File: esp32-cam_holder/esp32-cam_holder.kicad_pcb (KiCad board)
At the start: 2 copper layers, 28 x 55 mm, 6 parts, among them J1 RJ45_Shielded, J2 UART, U1 ESP32-CAM

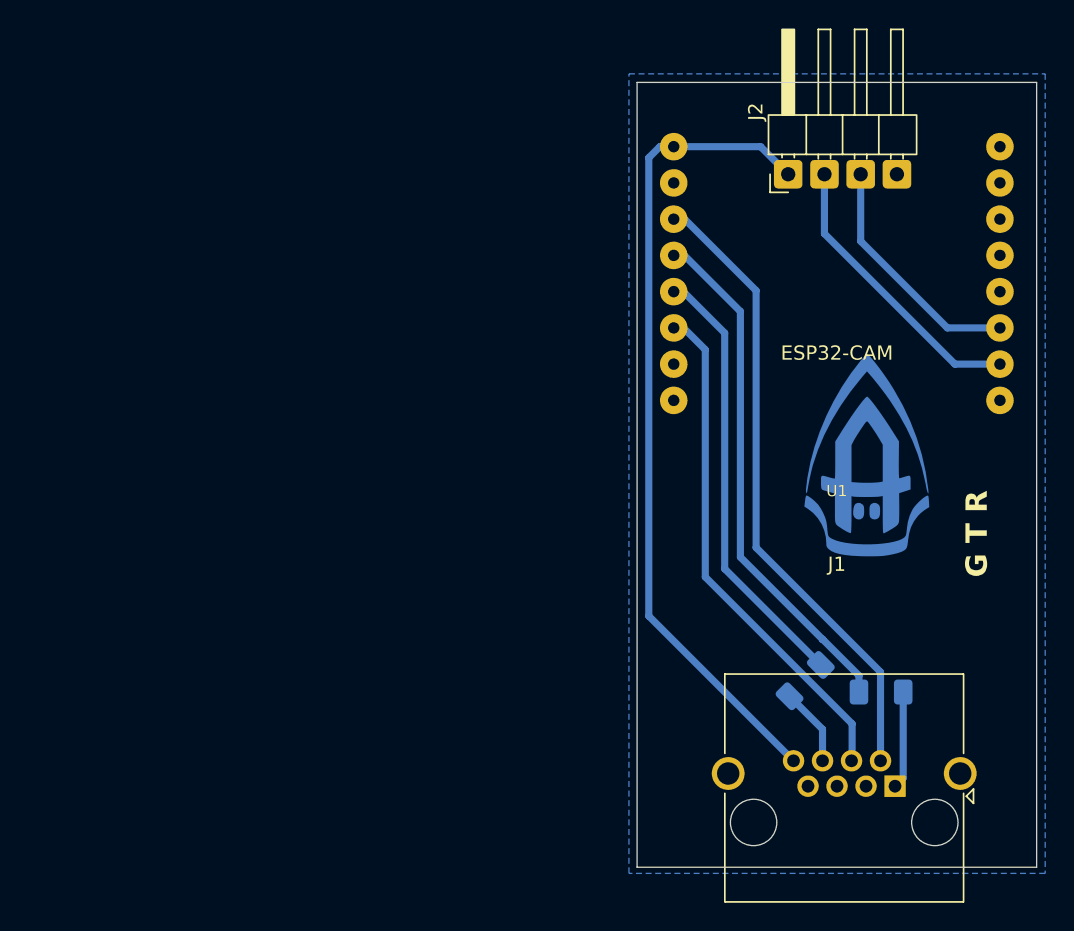
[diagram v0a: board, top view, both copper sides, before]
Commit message: REV ALL
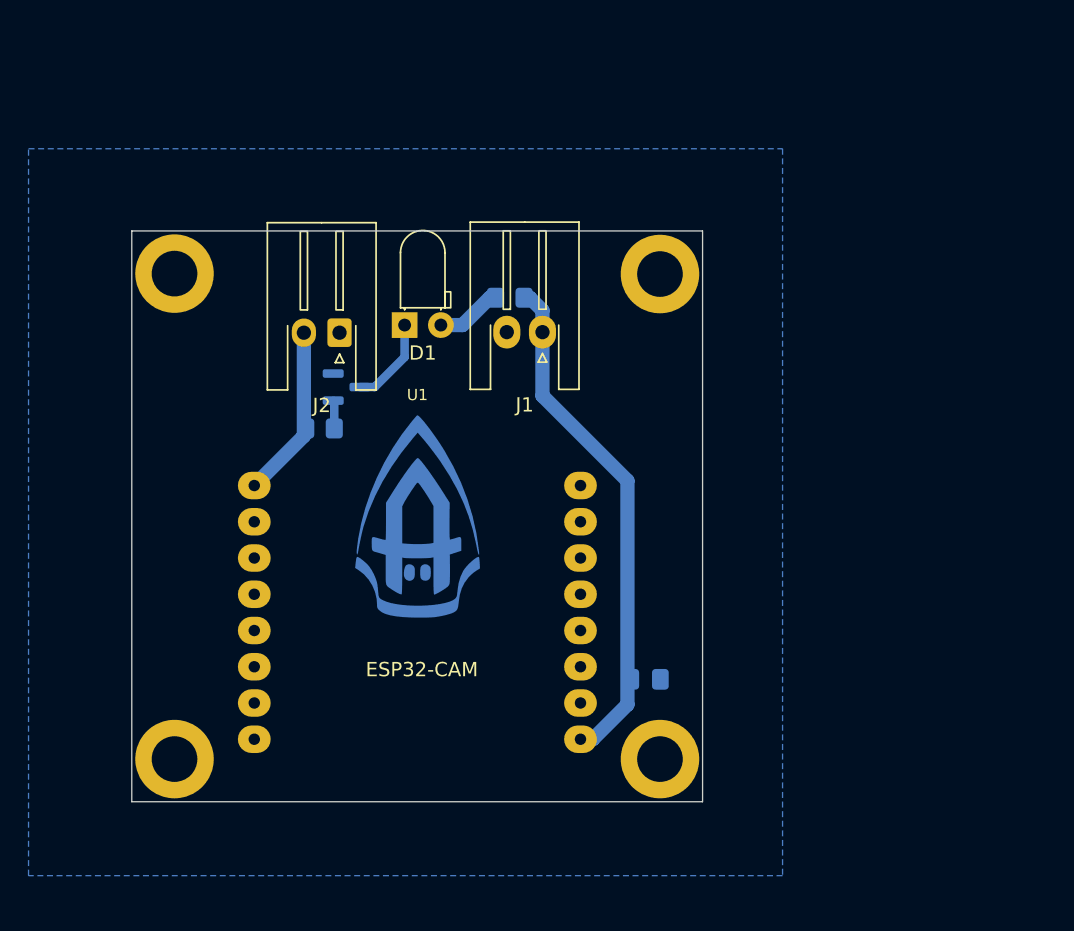
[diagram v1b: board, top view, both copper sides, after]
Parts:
- added C1: 100nF, Capacitor_SMD:C_0805_2012Metric_Pad1.18x1.45mm_HandSolder, B.Cu at (135.6, 57.1)
- added D1: LED, LED_THT:LED_D3.0mm_Horizontal_O1.27mm_Z6.0mm, F.Cu at (121.2, 32.3)
- added Q1: MMBT3904, Package_TO_SOT_SMD:SOT-23, B.Cu at (114.6, 36.7)
- added REF**: MountingHole_3.2mm_M3_ISO14580_Pad, MountingHole:MountingHole_3.2mm_M3_ISO14580_Pad, F.Cu at (102.6, 62.7)
- added REF**: MountingHole_3.2mm_M3_ISO14580_Pad, MountingHole:MountingHole_3.2mm_M3_ISO14580_Pad, F.Cu at (136.6, 62.7)
- added REF**: MountingHole_3.2mm_M3_ISO14580_Pad, MountingHole:MountingHole_3.2mm_M3_ISO14580_Pad, F.Cu at (136.6, 28.7)
- added REF**: MountingHole_3.2mm_M3_ISO14580_Pad, MountingHole:MountingHole_3.2mm_M3_ISO14580_Pad, F.Cu at (102.6, 28.7)
- J1: value RJ45_Shielded -> power; footprint Connector_RJ:RJ45_Amphenol_RJHSE5380 -> Connector_JST:JST_XH_S2B-XH-A-1_1x02_P2.50mm_Horizontal
- J2: value UART -> RST; footprint Connector_PinHeader_2.54mm:PinHeader_1x04_P2.54mm_Horizontal -> Connector_JST:JST_XH_S2B-XH-A-1_1x02_P2.50mm_Horizontal
- R1: value 0 -> 220; footprint Resistor_SMD:R_1206_3216Metric_Pad1.30x1.75mm_HandSolder -> Resistor_SMD:R_0805_2012Metric_Pad1.20x1.40mm_HandSolder
- R2: value 0 -> 1k; footprint Resistor_SMD:R_1206_3216Metric_Pad1.30x1.75mm_HandSolder -> Resistor_SMD:R_0805_2012Metric_Pad1.20x1.40mm_HandSolder
- moved R2 43.4 mm to (112.8, 39.6)
- moved J1 40.3 mm to (128.4, 32.8)
- moved R1 33.9 mm to (126.1, 30.4), turned to 180 degrees
- moved J2 33.3 mm to (114.2, 32.9), turned to 180 degrees
- moved G*** 31.8 mm to (119.6, 45.7)
- moved U1 30.2 mm to (119.6, 37.2), turned to 0 degrees
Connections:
- J1 pad 1: MOSI -> +5V
- J1 pad 2: MISO -> GND
- J2 pad 1: +5V -> GND
- J2 pad 2: TX -> RST
- R1 pad 1: Net-(R1-Pad1) -> +5V
- R1 pad 2: SS -> Net-(D1-A)
- R2 pad 1: Net-(R2-Pad1) -> RST
- R2 pad 2: MOSI -> Net-(Q1-B)
- U1 pad GND1: GND -> RST
- U1 pad GND2: unconnected-(U1-PadGND2) -> GND
- U1 pad IO13: Net-(R2-Pad1) -> MOSI
- U1 pad IO15: Net-(R1-Pad1) -> SS
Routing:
- net MISO: track 44.4 -> 0.00 mm
- net Net-(R2-Pad1): track 35.9 -> 0.00 mm
- net CLK: track 35.9 -> 0.00 mm
- net Net-(R1-Pad1): track 30.8 -> 0.00 mm
- net +5V: track 57.4 -> 36.0 mm
- net TX: track 20.3 -> 0.00 mm
- net RX: track 17.0 -> 0.00 mm
- net RST: track 0.00 -> 12.1 mm
- net MOSI: track 6.84 -> 0.00 mm
- net Net-(D1-K): track 0.00 -> 6.24 mm
- net SS: track 5.48 -> 0.00 mm
- net Net-(D1-A): track 0.00 -> 4.62 mm
- net Net-(Q1-B): track 0.00 -> 1.98 mm
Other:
- board size 28 x 55 mm -> 40 x 40 mm
- board text removed: "G T R"
